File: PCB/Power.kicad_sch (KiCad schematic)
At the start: 27 parts, among them J201 Barrel_Jack, Q201 BC847, Q202 BCV49, U201 LV3842, U202 LV3842

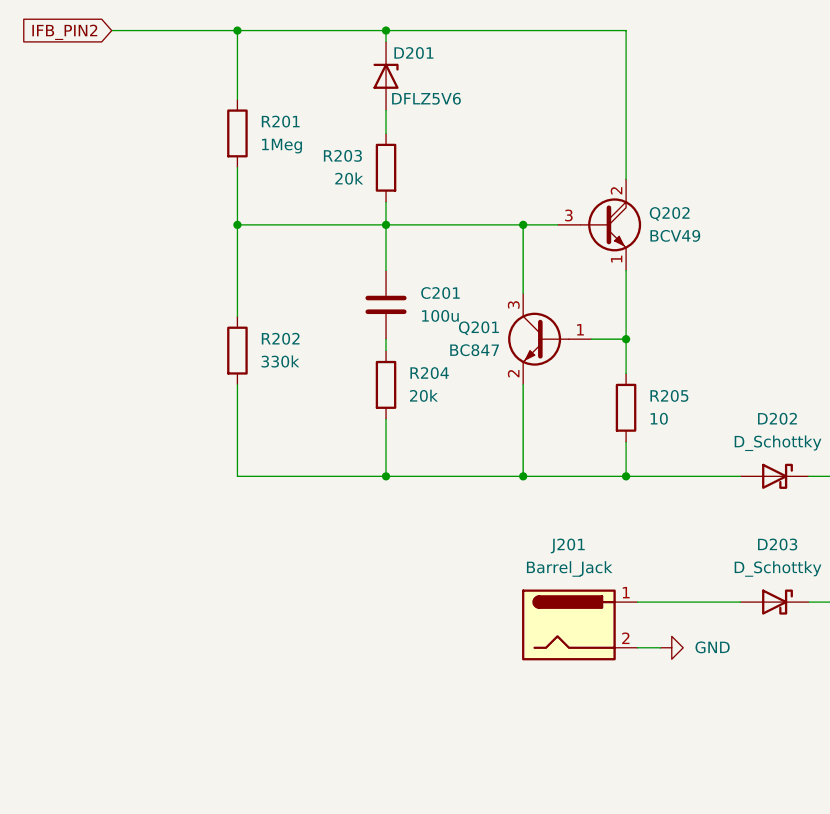
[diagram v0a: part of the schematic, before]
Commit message: Wooooooo
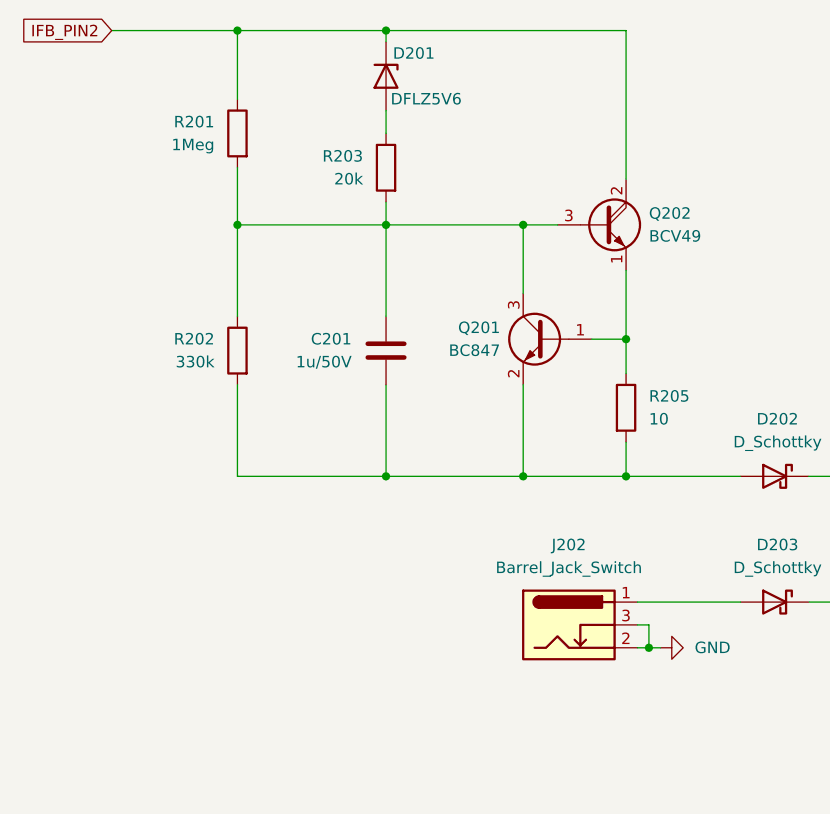
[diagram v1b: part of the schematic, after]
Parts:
- removed J201: Barrel_Jack, Connector_BarrelJack:BarrelJack_Horizontal, symbol Connector:Barrel_Jack
- removed R204: 20k, Resistor_SMD:R_0402_1005Metric, symbol Device:R
- added J202: Barrel_Jack_Switch, STEVEannouncer:Barrel Jack, symbol Connector:Barrel_Jack_Switch
- C201: value 100u -> 1u/50V; footprint (none) -> Capacitor_SMD:C_0402_1005Metric; Mouser Part Number (none) -> 81-GRM155R61H105KE5D
- C203, C204: footprint (none) -> Capacitor_SMD:C_0603_1608Metric; Mouser Part Number (none) -> 81-GRT188R61H225KE3D
- C205, C206: Mouser Part Number (none) -> 81-GRM155R62A104KE4D
- C207, C208: footprint (none) -> Capacitor_SMD:C_1206_3216Metric; Mouser Part Number (none) -> 791-1206X226K100CT
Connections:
- net GND: now also J202.2, J202.3
- net at C201.2: now also D202.2 (A), Q201.2 (E), R202.2, R205.2
- net at D203.2 (A): now also J202.1
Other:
- moved on the sheet: C201
